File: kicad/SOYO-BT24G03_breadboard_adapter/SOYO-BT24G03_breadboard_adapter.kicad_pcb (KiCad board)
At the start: 2 copper layers, 26.7 x 95.2 mm, 6 parts, among them J1 jack, P1 CONN_01X24, P2 CONN_01X24, P3 CONN_01X24, P4 CONN_01X24, U1 SOYO-BT24G03

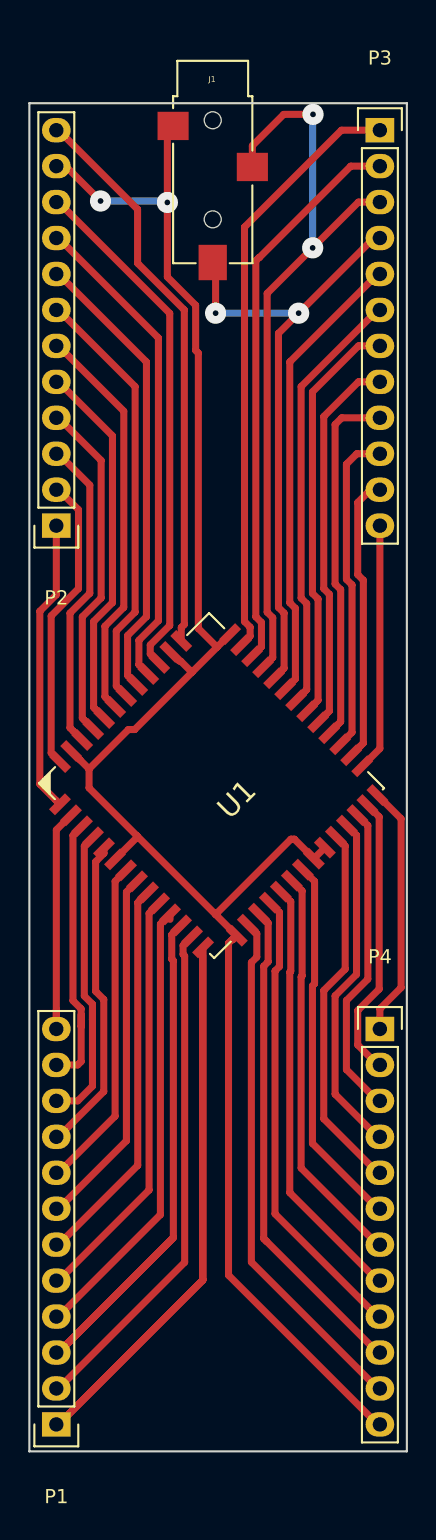
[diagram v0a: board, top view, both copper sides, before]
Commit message: update pcb,jack, layout
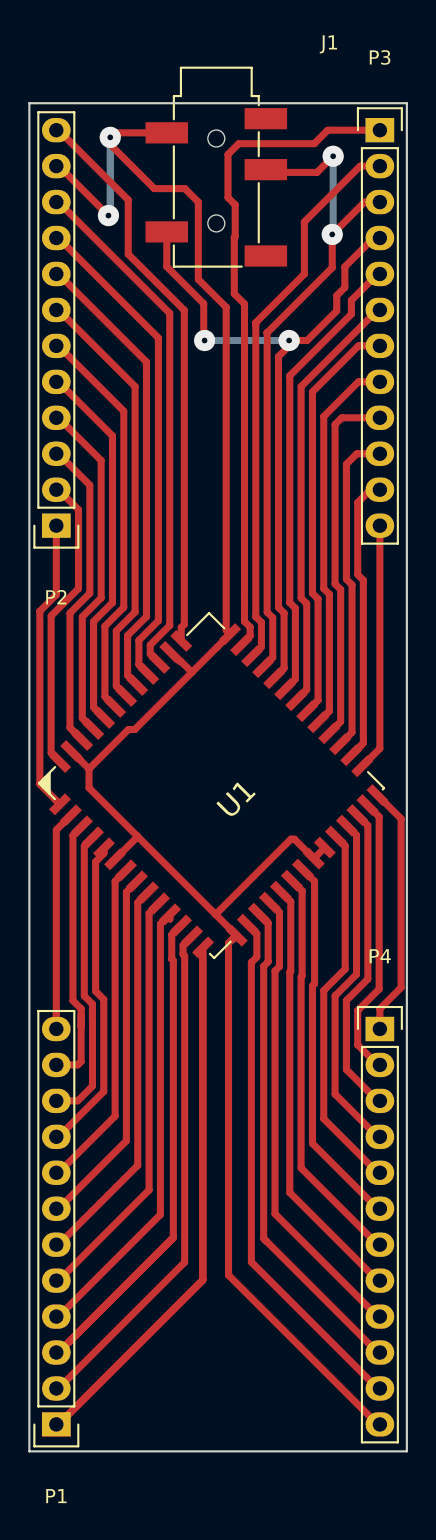
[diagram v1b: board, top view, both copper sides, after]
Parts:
- J1: footprint jacks:3.5mm_stereo_jack_PJ3026 -> jacks:PJ-327A
- moved J1 2.13 mm to (112.9, 30.6)
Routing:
- net Net-(J1-Pad1): track 133.9 -> 142.5 mm
- net Net-(J1-Pad5): track 44.3 -> 50.7 mm
- net Net-(P3-Pad1): track 42.7 -> 48.2 mm
- net Net-(J1-Pad2): track 53.8 -> 48.6 mm
